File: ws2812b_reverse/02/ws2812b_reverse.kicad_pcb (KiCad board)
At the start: 2 copper layers, 8.9 x 11.4 mm, 4 parts, among them J1 CONN_01X02, J2 CONN_01X02

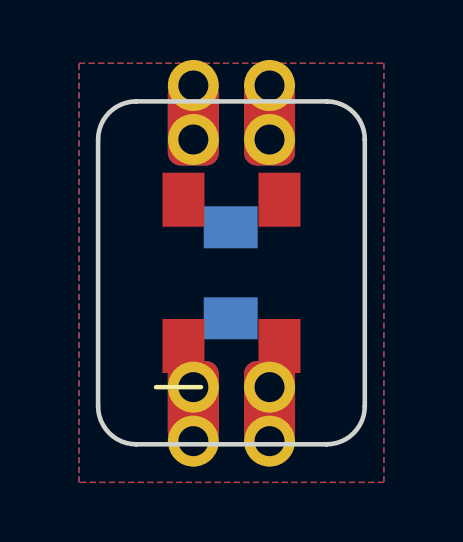
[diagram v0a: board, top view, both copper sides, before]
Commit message: Add Updates Neo Reverse
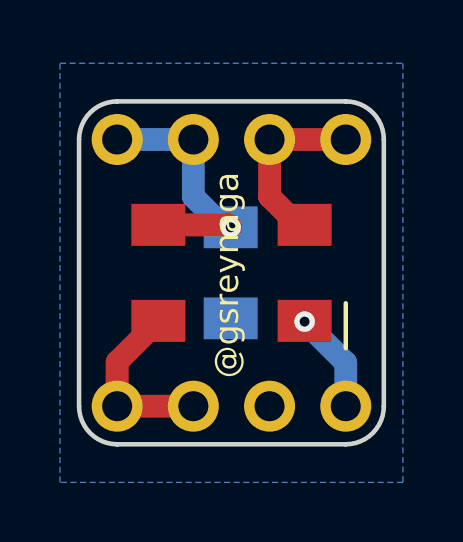
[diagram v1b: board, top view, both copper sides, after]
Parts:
- J1: value CONN_01X02 -> CONN_01X04; footprint neo-reverse:Pin_half-02x02_P2.54mm -> Connector_PinSocket_2.54mm:PinSocket_1x04_P2.54mm_WeMos; moved to F.Cu
- J2: value CONN_01X02 -> CONN_01X04; footprint neo-reverse:Pin_half-02x02_P2.54mm -> Connector_PinSocket_2.54mm:PinSocket_1x04_P2.54mm_WeMos
- moved J2 5.12 mm to (140.3, 111.8), turned to 90 degrees
- moved J1 5.08 mm to (140.3, 102.9)
- turned LED1 to 0 degrees
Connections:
- J1 pad 2: Net-(J1-Pad2) -> VCC
- J2 pad 2: GND -> Net-(J2-Pad1)
- LED1 pad 2: Net-(J1-Pad2) -> Net-(J1-Pad3)
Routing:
- net VCC: track 0.00 -> 8.56 mm, vias 0 -> 1
- net Net-(J1-Pad3): track 0.00 -> 6.00 mm
- net Net-(J2-Pad1): track 0.40 -> 5.95 mm
- net GND: track 0.55 -> 3.39 mm, vias 0 -> 1
- removed copper zone on F.Cu, net GND
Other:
- board size 8.9 x 11.4 mm -> 10.2 x 11.4 mm
- board text added: "@gsreynaga"
- board text added: "NEO"
- board text added: "REVERSE"
